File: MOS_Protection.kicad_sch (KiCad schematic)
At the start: 42 parts, among them Q10 PMOS, Q11 NMOS, Q12 NMOS, Q13 NMOS, Q14 NMOS, Q6 NMOS, Q7 NMOS, Q8 PMOS, Q9 NMOS

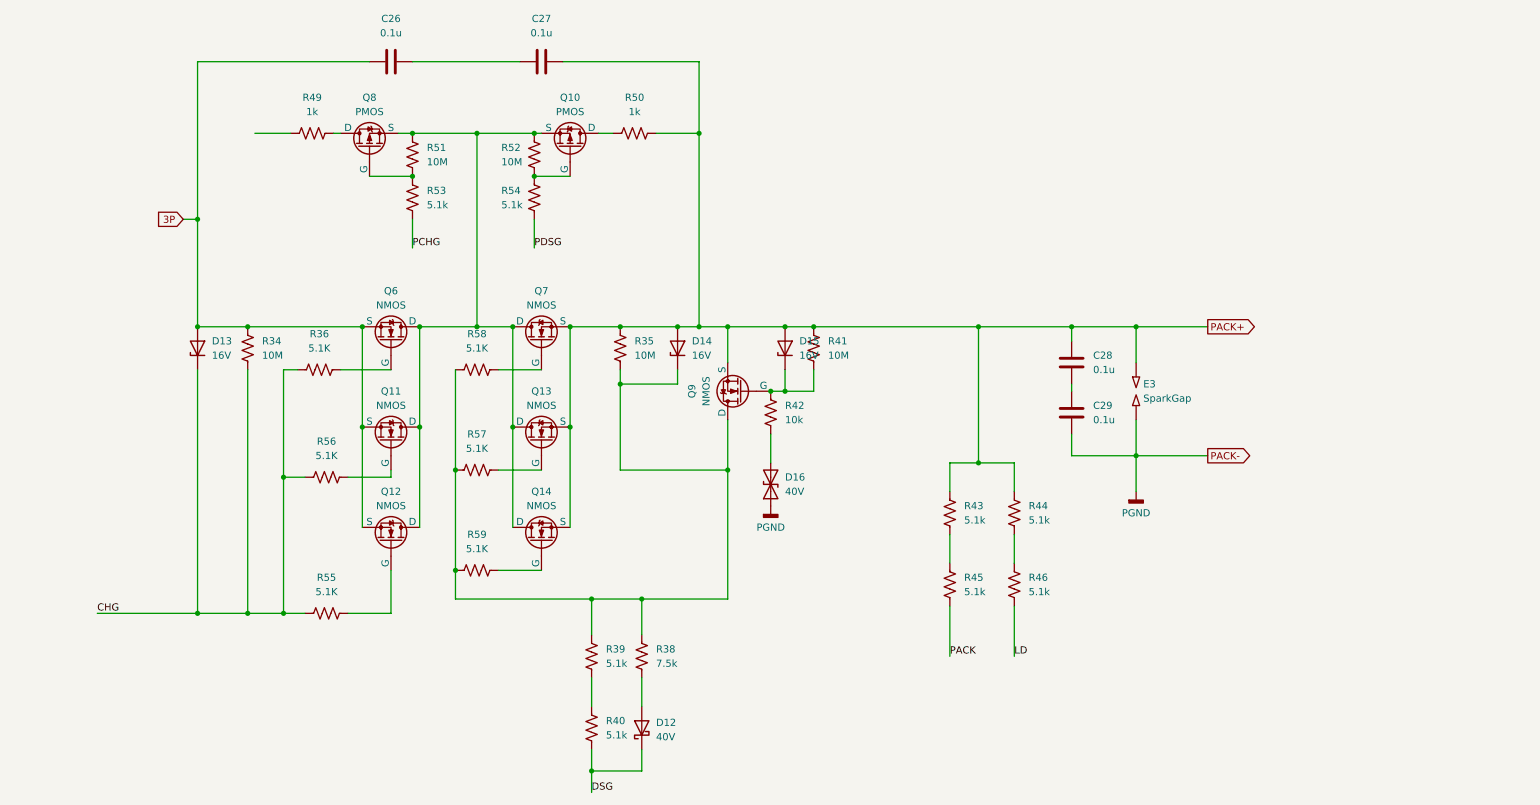
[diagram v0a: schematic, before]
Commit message: REV1 PCB that was sent to production (PCBWAY)
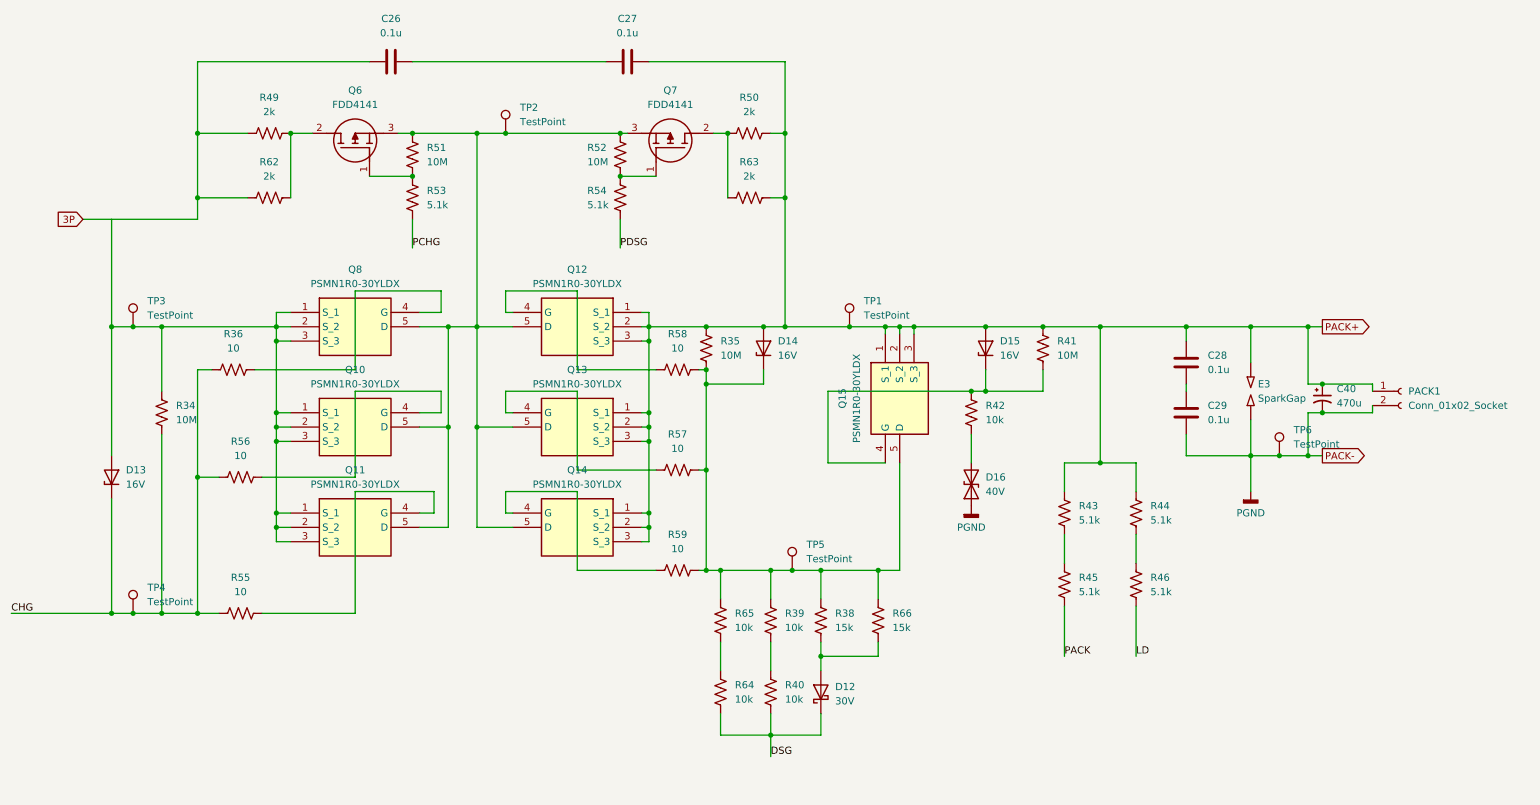
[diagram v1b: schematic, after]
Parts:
- removed Q10, Q8: PMOS, symbol Simulation_SPICE:PMOS
- removed Q11, Q12, Q13, Q14, Q6, Q7, Q9: NMOS, symbol Simulation_SPICE:NMOS
- added C40: 470u, Capacitor_SMD:C_Elec_8x10.2, symbol Device:C_Polarized_Small_US
- added PACK1: Conn_01x02_Socket, AMASS_github:AMASS_XT60-F_1x02_P7.20mm_Vertical, symbol Connector:Conn_01x02_Socket
- added Q10, Q11, Q12, Q13, Q14, Q15, Q8: PSMN1R0-30YLDX, SamacSys_Parts:PSMN5R660YLX, symbol SamacSys_Parts:PSMN1R0-30YLDX
- added Q6, Q7: FDD4141, SamacSys_Parts:FQD1N80TM, symbol SamacSys_Parts:FDD4141
- added R62, R63: 2k, Resistor_SMD:R_0805_2012Metric, symbol Device:R_US
- added R64, R65: 10k, Resistor_SMD:R_0805_2012Metric, symbol Device:R_US
- added R66: 15k, Resistor_SMD:R_0805_2012Metric, symbol Device:R_US
- added TP1, TP2, TP3, TP4, TP5, TP6: TestPoint, TestPoint:TestPoint_Pad_D1.0mm, symbol Connector:TestPoint
- C26, C27, C28, C29: footprint (none) -> Capacitor_SMD:C_0805_2012Metric
- D12: value 40V -> 30V; footprint (none) -> Diode_SMD:D_SOD-123
- D13, D14, D15, D16: footprint (none) -> Diode_SMD:D_SOD-123
- E3: footprint (none) -> Jumper:SolderJumper-2_P1.3mm_Open_TrianglePad1.0x1.5mm; now left out of the parts list
- R34, R35, R41, R42, R43, R44, R45, R46, R51, R52, R53, R54: footprint (none) -> Resistor_SMD:R_0805_2012Metric
- R36, R55, R56, R57, R58, R59: value 5.1K -> 10; footprint (none) -> Resistor_SMD:R_0805_2012Metric
- R38: value 7.5k -> 15k; footprint (none) -> Resistor_SMD:R_0805_2012Metric
- R39, R40: value 5.1k -> 10k; footprint (none) -> Resistor_SMD:R_0805_2012Metric
- R49, R50: value 1k -> 2k; footprint (none) -> Resistor_SMD:R_0805_2012Metric
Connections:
- net 3P: now also R49.1, R62.1; no longer D13.2 (A), R34.1
- net CHG: now also TP4.1
- net DSG: now also R64.2
- net PACK+: now also C40.1, PACK1.1 (Pin_1), Q12.1 (S_1), Q12.2 (S_2), Q12.3 (S_3), Q13.1 (S_1), Q13.2 (S_2), Q13.3 (S_3), Q14.1 (S_1), Q14.2 (S_2), Q14.3 (S_3), Q15.1 (S_1), Q15.2 (S_2), Q15.3 (S_3), R63.2, TP1.1
- net PGND: now also C40.2, PACK1.2 (Pin_2), TP6.1
- net at R51.1, R53.2: now also Q6.1 (G)
- net at R36.2: now also Q8.4 (G)
- net at R52.1, R54.2: now also Q7.1 (G)
- net at R51.2, R52.2: now also Q10.5 (D), Q11.5 (D), Q12.5 (D), Q13.5 (D), Q14.5 (D), Q6.3 (S), Q7.3 (S), Q8.5 (D), TP2.1
- net at D14.1 (K), R35.2, R38.1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: now also R57.2, R58.2, R59.2, Q15.5 (D), R65.1, R66.1, TP5.1; no longer R57.1, R58.1, R59.1
- net at R49.2: now also Q6.2 (D), R62.2
- net at D15.1 (K), R41.2, R42.1: now also Q15.4 (G)
- net at R55.2: now also Q11.4 (G)
- net at D12.2 (A), R38.2: now also R66.2
- net at R56.2: now also Q10.4 (G)
- net at R50.1: now also Q7.2 (D), R63.1
- new net: R64.1, R65.2
- new net: D13.2 (A), Q10.1 (S_1), Q10.2 (S_2), Q10.3 (S_3), Q11.1 (S_1), Q11.2 (S_2), Q11.3 (S_3), Q8.1 (S_1), Q8.2 (S_2), Q8.3 (S_3), R34.1, TP3.1
- new net: Q13.4 (G), R57.1
- new net: Q12.4 (G), R58.1
- new net: Q14.4 (G), R59.1
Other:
- moved on the sheet: C27, C28, C29, D12, D13, D14, D15, D16, E3, R34, R35, R36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
